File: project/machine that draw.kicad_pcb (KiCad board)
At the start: 2 copper layers, 53.1 x 84.4 mm, 25 parts, among them J1 SD_Card, J10 Screw_Terminal_01x02, J2 SSD1306 / 1 GND / 2 VCC / 3 S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, J3 limit switch_X, J4 limit switch_Y, J5 Motor_X, J6 motor_Y, J7 Barrel_Jack, J8 Conn_02x03_Odd_Even, J9 Conn_02x03_Odd_Even, U1 ESP32-S3-UNO, U2 Regulateur

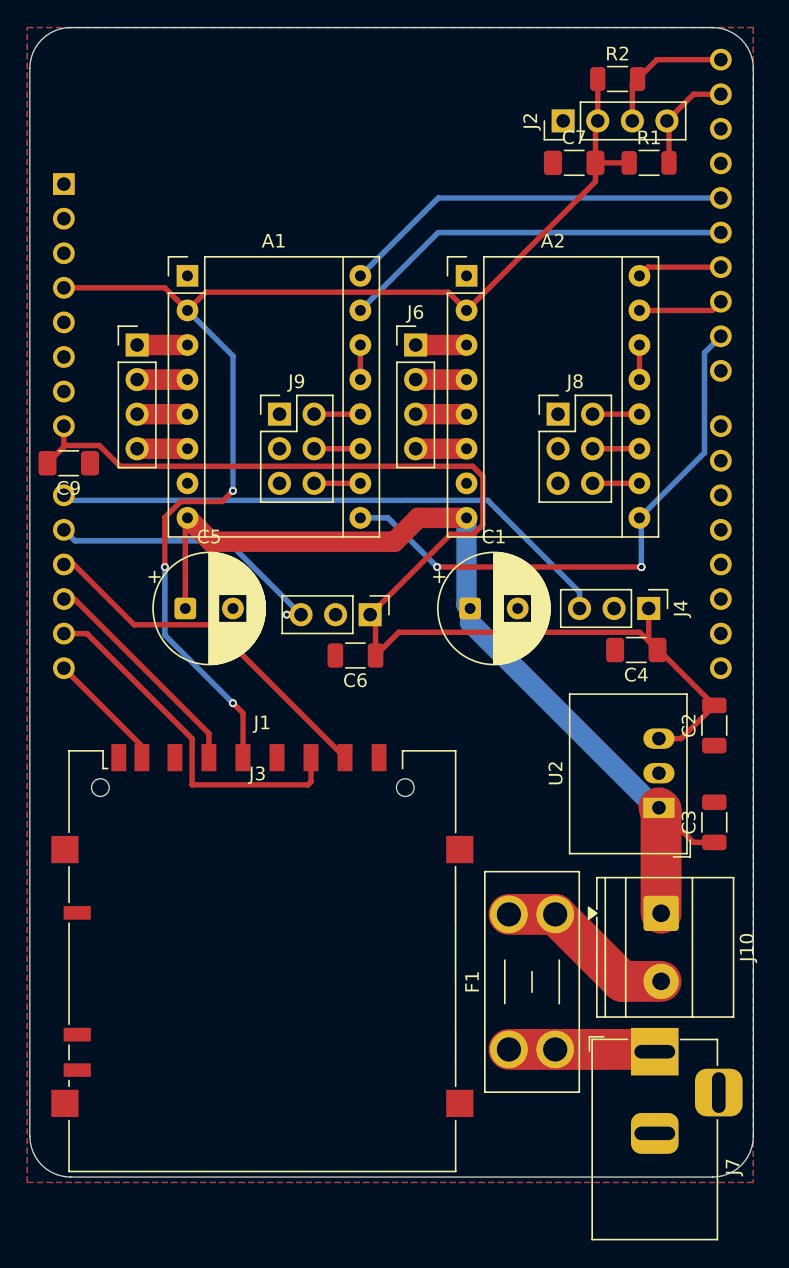
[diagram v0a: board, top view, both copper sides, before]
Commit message: fix wiring problems
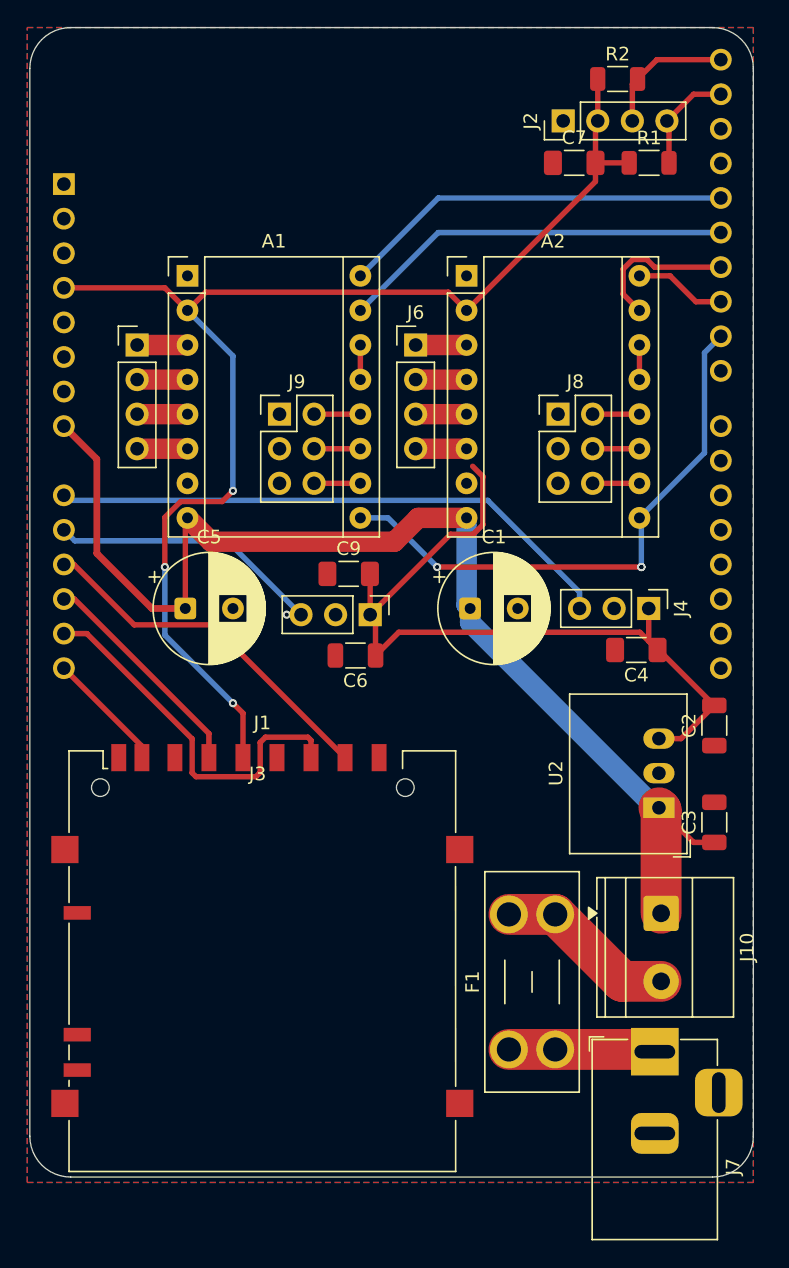
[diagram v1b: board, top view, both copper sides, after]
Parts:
- moved C9 22.1 mm to (143.5, 95.5), turned to 0 degrees
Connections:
- J7 pad 1: Net-(F1-Pad1) -> +12V
- U1 pad 25: STEP_Y -> DIR_Y
- U1 pad 26: DIR_Y -> STEP_Y
- U1 pad 8: +5V -> +12V
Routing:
- net +5V: track 88.9 -> 58.0 mm
- net +12V: track 69.7 -> 88.2 mm
- net STEP_Y: track 6.25 -> 11.2 mm
- net MOSI: track 26.6 -> 27.8 mm
- net DIR_Y: track 6.25 -> 6.77 mm
